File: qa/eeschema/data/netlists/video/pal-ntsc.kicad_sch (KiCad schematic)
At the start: 36 parts, among them U10 BT812, X2 30MHz

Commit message: Update netlist QA testcases to new file format
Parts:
- removed C1, C10, C11, C12, C13, C14, C2, C3, C4, C5, C6, C7, C8, C9: 100nF, Resistor_SMD:R_1206_3216Metric_Pad1.24x1.80mm_HandSolder, symbol video_schlib:C
- removed C47: 220pF, Resistor_SMD:R_1206_3216Metric_Pad1.24x1.80mm_HandSolder, symbol video_schlib:C
- removed C62: 47uF, Resistor_SMD:R_1210_3225Metric_Pad1.24x2.70mm_HandSolder, symbol video_schlib:CP
- removed C65, C66: 22pF, Resistor_SMD:R_1206_3216Metric_Pad1.24x1.80mm_HandSolder, symbol video_schlib:C
- removed D1, D2, D3, D4: BAT46, Diode_THT:D_DO-34_SOD68_P7.62mm_Horizontal, symbol video_schlib:DIODESCH
- removed L4: 22uF, Resistor_SMD:R_1812_4532Metric_Pad1.24x3.50mm_HandSolder, symbol video_schlib:INDUCTOR
- removed R12: 1K, Resistor_SMD:R_1206_3216Metric_Pad1.24x1.80mm_HandSolder, symbol video_schlib:R
- removed R14: 1M, Resistor_SMD:R_1206_3216Metric_Pad1.24x1.80mm_HandSolder, symbol video_schlib:R
- removed R19, R20: 220, Resistor_SMD:R_1206_3216Metric_Pad1.24x1.80mm_HandSolder, symbol video_schlib:R
- removed R2, R3: 100, Resistor_SMD:R_1206_3216Metric_Pad1.24x1.80mm_HandSolder, symbol video_schlib:R
- removed R25: 220K, Resistor_SMD:R_1206_3216Metric_Pad1.24x1.80mm_HandSolder, symbol video_schlib:R
- removed R27: 27K, Resistor_SMD:R_1206_3216Metric_Pad1.24x1.80mm_HandSolder, symbol video_schlib:R
- removed R35: 470, Resistor_SMD:R_1206_3216Metric_Pad1.24x1.80mm_HandSolder, symbol video_schlib:R
- removed X2: 30MHz, Crystal:Crystal_HC18-U_Vertical, symbol video_schlib:CRYSTAL
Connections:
- net C-VIDEO: now also U10.1 (VAA), U10.2 (VAA)
- net GND: now also U10.1 (VAA), U10.2 (VAA)
- net GREEN_IN: now also U10.2 (VAA)
- net RED_IN: now also U10.2 (VAA)
- net VCC: now also U10.1 (VAA), U10.2 (VAA)
- net Y-VIDEO: now also U10.1 (VAA), U10.2 (VAA)
- net Y_SYNC: now also U10.2 (VAA)
- net at U10.117 (VIN_C): now also U10.1 (VAA)
- net at U10.140 (SYNC_DET): now also U10.1 (VAA), U10.2 (VAA)
- net at U10.108 (XTAL1_IN): now also U10.1 (VAA), U10.2 (VAA)
- net at U10.109 (XTAL1_OUT): now also U10.1 (VAA), U10.2 (VAA)
- net at U10.113 (REFOUT), U10.137 (CREF+), U10.144 (YREF+): now also U10.1 (VAA)
- net at U10.114 (CLEVEL): now also U10.1 (VAA), U10.2 (VAA)
- net at U10.115 (OUT_C): now also U10.2 (VAA)
- net at U10.135 (R/2): now also U10.1 (VAA)
- net at U10.4 (VIN_Y/COMP.): now also U10.1 (VAA)
- new net: U10.1 (VAA), U10.2 (VAA) (x4)
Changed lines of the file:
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@@
-(kicad_sch (version 20200310) (host eeschema "(5.99.0-1545-g9916f24fa)")
-  (page "A3")
+(kicad_sch (version 20200512) (host eeschema "(5.99.0-1712-g5a9e69b14)")
+  (page 2 8)
+  (paper "A3")
   (title_block
     (title "Video")
@@
     (company "Kicad EDA")
   )
+  (junction (at 81.28 165.1))
+  (junction (at 101.6 165.1))
+  (junction (at 113.03 93.98))
+  (junction (at 113.03 106.68))
+  (junction (at 113.03 129.54))
+  (junction (at 113.03 142.24))
+  (junction (at 123.19 53.34))
+  (junction (at 123.19 66.04))
+  (junction (at 130.81 162.56))
+  (junction (at 143.51 53.34))
+  (junction (at 143.51 66.04))
+  (junction (at 148.59 154.94))
+  (junction (at 148.59 165.1))
+  (junction (at 148.59 175.26))
+  (junction (at 149.86 96.52))
+  (junction (at 149.86 104.14))
+  (junction (at 149.86 106.68))
+  (junction (at 161.29 60.96))
+  (junction (at 161.29 248.92))
+  (junction (at 163.83 60.96))
+  (junction (at 163.83 248.92))
+  (junction (at 166.37 60.96))
+  (junction (at 166.37 248.92))
+  (junction (at 168.91 60.96))
+  (junction (at 168.91 248.92))
+  (junction (at 171.45 60.96))
+  (junction (at 171.45 248.92))
+  (junction (at 173.99 60.96))
+  (junction (at 173.99 248.92))
+  (junction (at 176.53 248.92))
+  (junction (at 179.07 248.92))
+  (junction (at 189.23 60.96))
+  (junction (at 189.23 248.92))
+  (junction (at 191.77 60.96))
+  (junction (at 191.77 248.92))
+  (junction (at 194.31 60.96))
+  (junction (at 194.31 248.92))
+  (junction (at 196.85 60.96))
+  (junction (at 196.85 248.92))
+  (junction (at 199.39 60.96))
+  (junction (at 199.39 248.92))
+  (junction (at 201.93 60.96))
+  (junction (at 201.93 248.92))
+  (junction (at 204.47 60.96))
+  (junction (at 204.47 248.92))
+  (junction (at 207.01 60.96))
+  (junction (at 207.01 248.92))
+  (junction (at 209.55 60.96))
+  (junction (at 209.55 248.92))
+  (junction (at 212.09 60.96))
+  (junction (at 212.09 248.92))
+  (junction (at 214.63 60.96))
   (junction (at 214.63 248.92))
-  (junction (at 168.91 60.96))
+  (junction (at 217.17 60.96))
+  (junction (at 217.17 248.92))
+  (junction (at 219.71 60.96))
+  (junction (at 219.71 248.92))
+  (junction (at 222.25 60.96))
+  (junction (at 222.25 248.92))
+  (junction (at 224.79 60.96))
+  (junction (at 224.79 248.92))
+  (junction (at 227.33 60.96))
+  (junction (at 227.33 248.92))
+  (junction (at 229.87 60.96))
+  (junction (at 232.41 60.96))
+  (junction (at 234.95 60.96))
+  (junction (at 237.49 60.96))
   (junction (at 240.03 60.96))
-  (junction (at 349.25 231.14))
-  (junction (at 173.99 248.92))
-  (junction (at 199.39 248.92))
-  (junction (at 189.23 248.92))
-  (junction (at 367.03 218.44))
-  (junction (at 191.77 60.96))
-  (junction (at 234.95 60.96))
-  (junction (at 113.03 106.68))
-  (junction (at 168.91 248.92))
-  (junction (at 339.09 88.9))
-  (junction (at 321.31 88.9))
-  (junction (at 173.99 60.96))
-  (junction (at 209.55 60.96))
-  (junction (at 189.23 60.96))
   (junction (at 242.57 60.96))
   (junction (at 245.11 60.96))
+  (junction (at 273.05 45.72))
+  (junction (at 303.53 76.2))
+  (junction (at 303.53 88.9))
+  (junction (at 321.31 76.2))
+  (junction (at 321.31 88.9))
+  (junction (at 331.47 218.44))
+  (junction (at 331.47 231.14))
   (junction (at 339.09 76.2))
-  (junction (at 196.85 248.92))
-  (junction (at 303.53 76.2))
-  (junction (at 224.79 248.92))
-  (junction (at 196.85 60.96))
-  (junction (at 194.31 60.96))
-  (junction (at 273.05 45.72))
-  (junction (at 113.03 142.24))
-  (junction (at 161.29 248.92))
-  (junction (at 331.47 231.14))
-  (junction (at 179.07 248.92))
-  (junction (at 222.25 60.96))
-  (junction (at 113.03 93.98))
-  (junction (at 130.81 162.56))
-  (junction (at 194.31 248.92))
-  (junction (at 101.6 165.1))
-  (junction (at 143.51 53.34))
-  (junction (at 224.79 60.96))
-  (junction (at 166.37 60.96))
-  (junction (at 176.53 248.92))
-  (junction (at 303.53 88.9))
-  (junction (at 212.09 60.96))
-  (junction (at 171.45 248.92))
-  (junction (at 212.09 248.92))
-  (junction (at 149.86 104.14))
-  (junction (at 209.55 248.92))
+  (junction (at 339.09 88.9))
   (junction (at 349.25 218.44))
-  (junction (at 207.01 248.92))
-  (junction (at 321.31 76.2))
-  (junction (at 163.83 248.92))
-  (junction (at 204.47 248.92))
-  (junction (at 161.29 60.96))
-  (junction (at 219.71 248.92))
-  (junction (at 123.19 53.34))
-  (junction (at 149.86 106.68))
-  (junction (at 148.59 175.26))
-  (junction (at 217.17 60.96))
-  (junction (at 222.25 248.92))
-  (junction (at 201.93 248.92))
-  (junction (at 331.47 218.44))
-  (junction (at 191.77 248.92))
+  (junction (at 349.25 231.14))
+  (junction (at 367.03 218.44))
   (junction (at 367.03 231.14))
-  (junction (at 199.39 60.96))
-  (junction (at 148.59 165.1))
-  (junction (at 143.51 66.04))
-  (junction (at 81.28 165.1))
-  (junction (at 149.86 96.52))
-  (junction (at 219.71 60.96))
-  (junction (at 171.45 60.96))
-  (junction (at 232.41 60.96))
-  (junction (at 217.17 248.92))
-  (junction (at 166.37 248.92))
-  (junction (at 227.33 60.96))
-  (junction (at 123.19 66.04))
-  (junction (at 229.87 60.96))
-  (junction (at 113.03 129.54))
-  (junction (at 204.47 60.96))
-  (junction (at 201.93 60.96))
-  (junction (at 148.59 154.94))
-  (junction (at 214.63 60.96))
-  (junction (at 163.83 60.96))
-  (junction (at 237.49 60.96))
-  (junction (at 227.33 248.92))
-  (junction (at 207.01 60.96))
   (no_connect (at 151.13 91.44))
   (no_connect (at 151.13 134.62))
+  (no_connect (at 255.27 200.66))
+  (no_connect (at 255.27 177.8))
+  (no_connect (at 255.27 175.26))
+  (no_connect (at 151.13 111.76))
+  (no_connect (at 151.13 124.46))
+  (no_connect (at 151.13 127))
+  (no_connect (at 255.27 218.44))
+  (no_connect (at 151.13 142.24))
+  (no_connect (at 255.27 205.74))
   (no_connect (at 151.13 88.9))
+  (no_connect (at 255.27 198.12))
+  (no_connect (at 255.27 182.88))
+  (no_connect (at 255.27 208.28))
+  (no_connect (at 151.13 132.08))
+  (no_connect (at 151.13 139.7))
+  (no_connect (at 255.27 210.82))
   (no_connect (at 255.27 195.58))
-  (no_connect (at 151.13 132.08))
   (no_connect (at 255.27 180.34))
-  (no_connect (at 151.13 111.76))
-  (no_connect (at 151.13 127))
-  (no_connect (at 255.27 210.82))
-  (no_connect (at 151.13 142.24))
-  (no_connect (at 255.27 177.8))
-  (no_connect (at 255.27 200.66))
-  (no_connect (at 151.13 124.46))
-  (no_connect (at 255.27 205.74))
-  (no_connect (at 151.13 139.7))
-  (no_connect (at 255.27 175.26))
-  (no_connect (at 255.27 182.88))
-  (no_connect (at 255.27 198.12))
-  (no_connect (at 255.27 218.44))
-  (no_connect (at 255.27 208.28))
   (bus_entry (at 267.97 81.28) (size 2.54 -2.54))
   (bus_entry (at 267.97 83.82) (size 2.54 -2.54))

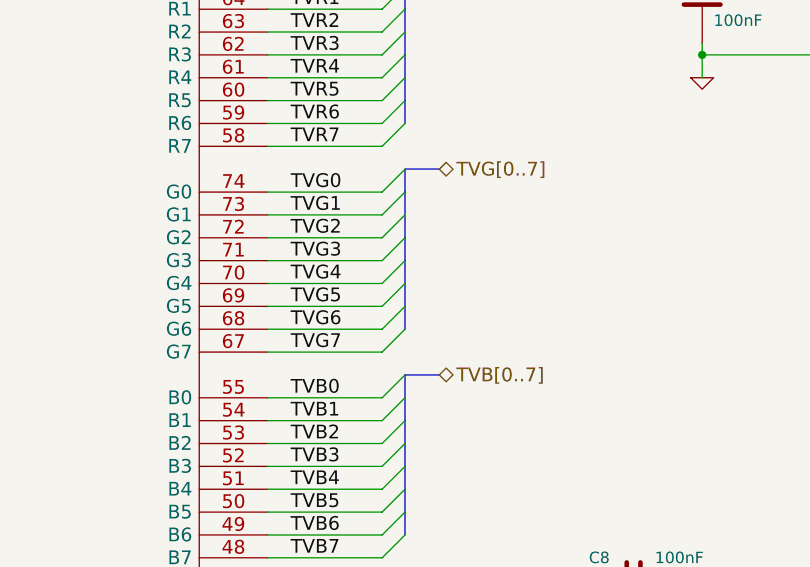
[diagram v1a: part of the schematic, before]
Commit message: Convert video QA project to new format
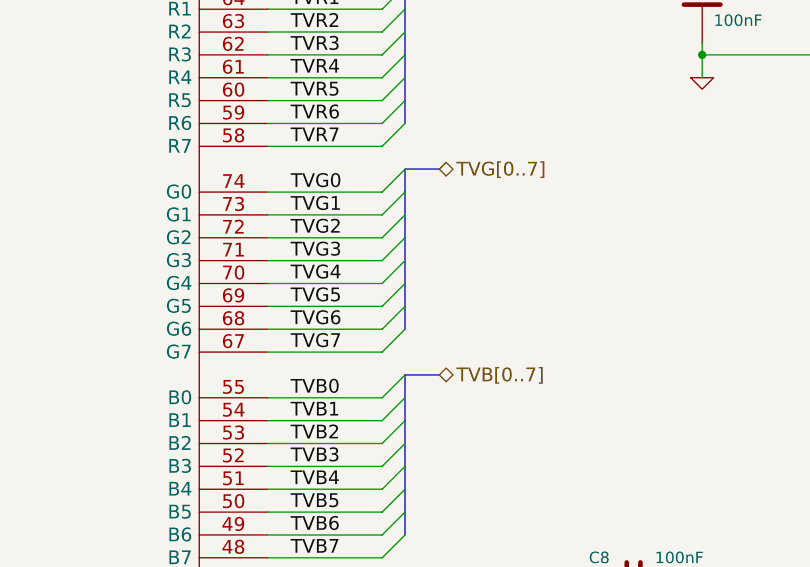
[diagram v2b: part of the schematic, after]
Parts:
- added C1, C10, C11, C12, C13, C14, C2, C3, C4, C5, C6, C7, C8, C9: 100nF, Resistor_SMD:R_1206_3216Metric_Pad1.24x1.80mm_HandSolder, symbol video_schlib:C
- added C47: 220pF, Resistor_SMD:R_1206_3216Metric_Pad1.24x1.80mm_HandSolder, symbol video_schlib:C
- added C62: 47uF, Resistor_SMD:R_1210_3225Metric_Pad1.24x2.70mm_HandSolder, symbol video_schlib:CP
- added C65, C66: 22pF, Resistor_SMD:R_1206_3216Metric_Pad1.24x1.80mm_HandSolder, symbol video_schlib:C
- added D1, D2, D3, D4: BAT46, Diode_THT:D_DO-34_SOD68_P7.62mm_Horizontal, symbol video_schlib:DIODESCH
- added L4: 22uF, Resistor_SMD:R_1812_4532Metric_Pad1.24x3.50mm_HandSolder, symbol video_schlib:INDUCTOR
- added R12: 1K, Resistor_SMD:R_1206_3216Metric_Pad1.24x1.80mm_HandSolder, symbol video_schlib:R
- added R14: 1M, Resistor_SMD:R_1206_3216Metric_Pad1.24x1.80mm_HandSolder, symbol video_schlib:R
- added R19, R20: 220, Resistor_SMD:R_1206_3216Metric_Pad1.24x1.80mm_HandSolder, symbol video_schlib:R
- added R2, R3: 100, Resistor_SMD:R_1206_3216Metric_Pad1.24x1.80mm_HandSolder, symbol video_schlib:R
- added R25: 220K, Resistor_SMD:R_1206_3216Metric_Pad1.24x1.80mm_HandSolder, symbol video_schlib:R
- added R27: 27K, Resistor_SMD:R_1206_3216Metric_Pad1.24x1.80mm_HandSolder, symbol video_schlib:R
- added R35: 470, Resistor_SMD:R_1206_3216Metric_Pad1.24x1.80mm_HandSolder, symbol video_schlib:R
- added X2: 30MHz, Crystal:Crystal_HC18-U_Vertical, symbol video_schlib:CRYSTAL
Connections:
- net C-VIDEO: now also D3.2 (K), D4.1 (A), R2.1; no longer U10.1 (VAA), U10.2 (VAA)
- net GND: now also C10.2, C11.2, C12.2, C13.2, C14.2, C2.2, C47.2, C6.2, C62.2, C65.1, C66.1, C7.2, C9.2, D1.1 (A), D3.1 (A), R14.2; no longer U10.1 (VAA), U10.2 (VAA)
- net GREEN_IN: now also C3.2; no longer U10.2 (VAA)
- net RED_IN: now also C4.2; no longer U10.2 (VAA)
- net VAF: now also C12.1, C13.1, C14.1, C2.1, C62.1, L4.2, R12.2
- net VCC: now also C10.1, C11.1, C9.1, D2.2 (K), D4.2 (K), L4.1; no longer U10.1 (VAA), U10.2 (VAA)
- net Y-VIDEO: now also D1.2 (K), D2.1 (A), R3.1; no longer U10.1 (VAA), U10.2 (VAA)
- net Y_SYNC: now also R20.2, R35.2; no longer U10.2 (VAA)
- net at U10.113 (REFOUT), U10.137 (CREF+), U10.144 (YREF+): now also C6.1, R12.1; no longer U10.1 (VAA)
- net at U10.117 (VIN_C): now also C5.1; no longer U10.1 (VAA)
- net at U10.135 (R/2): now also R27.1; no longer U10.1 (VAA)
- net at U10.4 (VIN_Y/COMP.): now also C8.1; no longer U10.1 (VAA)
- net at U10.115 (OUT_C): now also R19.2; no longer U10.2 (VAA)
- new net: C1.1, C47.1, R35.1
- new net: C7.1, R27.2, U10.114 (CLEVEL)
- new net: C65.2, R25.2, U10.109 (XTAL1_OUT), X2.1
- new net: C5.2, R19.1
- new net: C66.2, R25.1, U10.108 (XTAL1_IN), X2.2
- new net: C8.2, R20.1
- new net: C1.2, R14.1, U10.140 (SYNC_DET)
- new net: C4.1, R2.2
- new net: C3.1, R3.2
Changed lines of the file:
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@@
-(kicad_sch (version 20200512) (host eeschema "(5.99.0-1712-g5a9e69b14)")
-  (page 2 8)
+(kicad_sch (version 20200512) (host eeschema "(5.99.0-1722-g89c46e683-dirty)")
+  (page 1 8)
   (paper "A3")
   (title_block
@@
   (junction (at 367.03 218.44))
   (junction (at 367.03 231.14))
+  (no_connect (at 255.27 200.66))
+  (no_connect (at 255.27 195.58))
+  (no_connect (at 151.13 142.24))
+  (no_connect (at 255.27 210.82))
+  (no_connect (at 151.13 127))
+  (no_connect (at 255.27 180.34))
+  (no_connect (at 255.27 177.8))
+  (no_connect (at 255.27 198.12))
+  (no_connect (at 151.13 124.46))
+  (no_connect (at 151.13 111.76))
+  (no_connect (at 255.27 175.26))
+  (no_connect (at 255.27 205.74))
+  (no_connect (at 151.13 132.08))
+  (no_connect (at 151.13 139.7))
+  (no_connect (at 151.13 88.9))
+  (no_connect (at 255.27 182.88))
+  (no_connect (at 255.27 218.44))
+  (no_connect (at 255.27 208.28))
   (no_connect (at 151.13 91.44))
   (no_connect (at 151.13 134.62))
-  (no_connect (at 255.27 200.66))
-  (no_connect (at 255.27 177.8))
-  (no_connect (at 255.27 175.26))
-  (no_connect (at 151.13 111.76))
-  (no_connect (at 151.13 124.46))
-  (no_connect (at 151.13 127))
-  (no_connect (at 255.27 218.44))
-  (no_connect (at 151.13 142.24))
-  (no_connect (at 255.27 205.74))
-  (no_connect (at 151.13 88.9))
-  (no_connect (at 255.27 198.12))
-  (no_connect (at 255.27 182.88))
-  (no_connect (at 255.27 208.28))
-  (no_connect (at 151.13 132.08))
-  (no_connect (at 151.13 139.7))
-  (no_connect (at 255.27 210.82))
-  (no_connect (at 255.27 195.58))
-  (no_connect (at 255.27 180.34))
   (bus_entry (at 267.97 81.28) (size 2.54 -2.54))
   (bus_entry (at 267.97 83.82) (size 2.54 -2.54))
@@
   (bus (pts (xy 270.51 101.6) (xy 270.51 104.14)))
   (bus (pts (xy 270.51 104.14) (xy 270.51 109.22)))
-  (bus (pts (xy 270.51 109.22) (xy 270.51 111.76)))
-  (bus (pts (xy 270.51 111.76) (xy 270.51 116.84)))
-  (bus (pts (xy 270.51 116.84) (xy 270.51 119.38)))
+  (bus (pts (xy 270.51 109.22) (xy 270.51 114.3)))
+  (bus (pts (xy 270.51 114.3) (xy 270.51 119.38)))
   (bus (pts (xy 270.51 124.46) (xy 270.51 129.54)))
   (bus (pts (xy 270.51 129.54) (xy 270.51 134.62)))
